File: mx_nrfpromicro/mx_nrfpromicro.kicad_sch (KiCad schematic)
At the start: 21 parts, among them J1 Conn_01x02, SW1 SW_Push_45deg, SW10 SW_Push_45deg, SW11 SW_Push_45deg, SW12 SW_Push_45deg, SW13 SW_Push_45deg, SW14 SW_Push_45deg, SW15 SW_Push_45deg, SW16 SW_Push_45deg, SW17 SW_Push_45deg, SW18 SW_Push, SW2 SW_Push_45deg, SW3 SW_Push_45deg, SW4 SW_Push_45deg, SW5 SW_Push_45deg, SW6 SW_Push_45deg, SW7 SW_Push_45deg, SW8 SW_Push_45deg, SW9 SW_Push_45deg, U1 Nice_Nano_V2

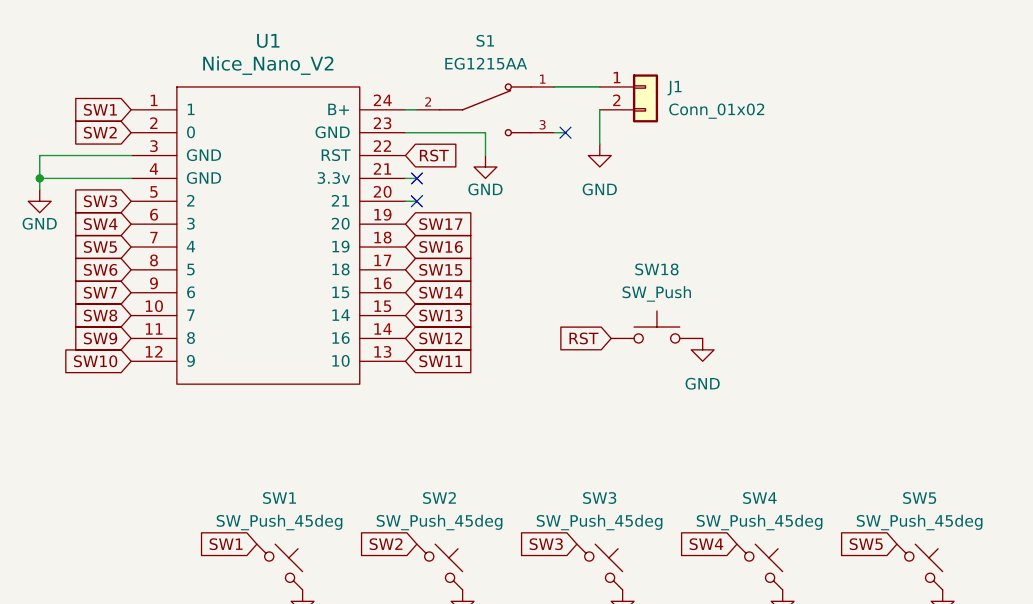
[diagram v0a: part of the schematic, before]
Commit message: updated
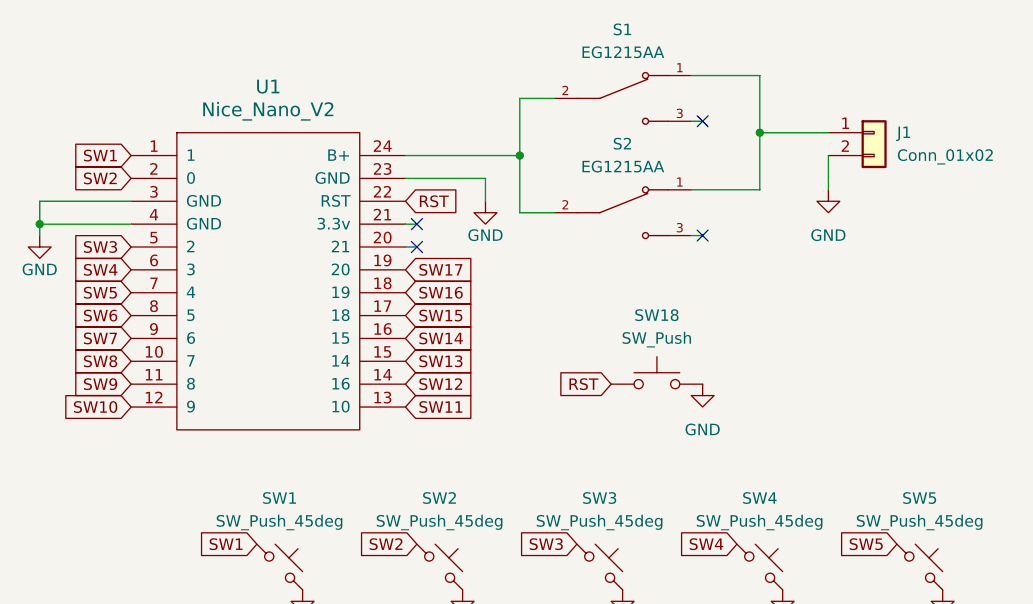
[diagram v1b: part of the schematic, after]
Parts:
- added S2: EG1215AA, EG1215AA:SW_EG1215AA, symbol EG1215AA:EG1215AA
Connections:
- net at S1.2, U1.24 (B+): now also S2.2
- net at J1.1 (Pin_1), S1.1: now also S2.1
- no-connect marks 3 -> 4
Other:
- moved on the sheet: J1, S1, SW18, U1

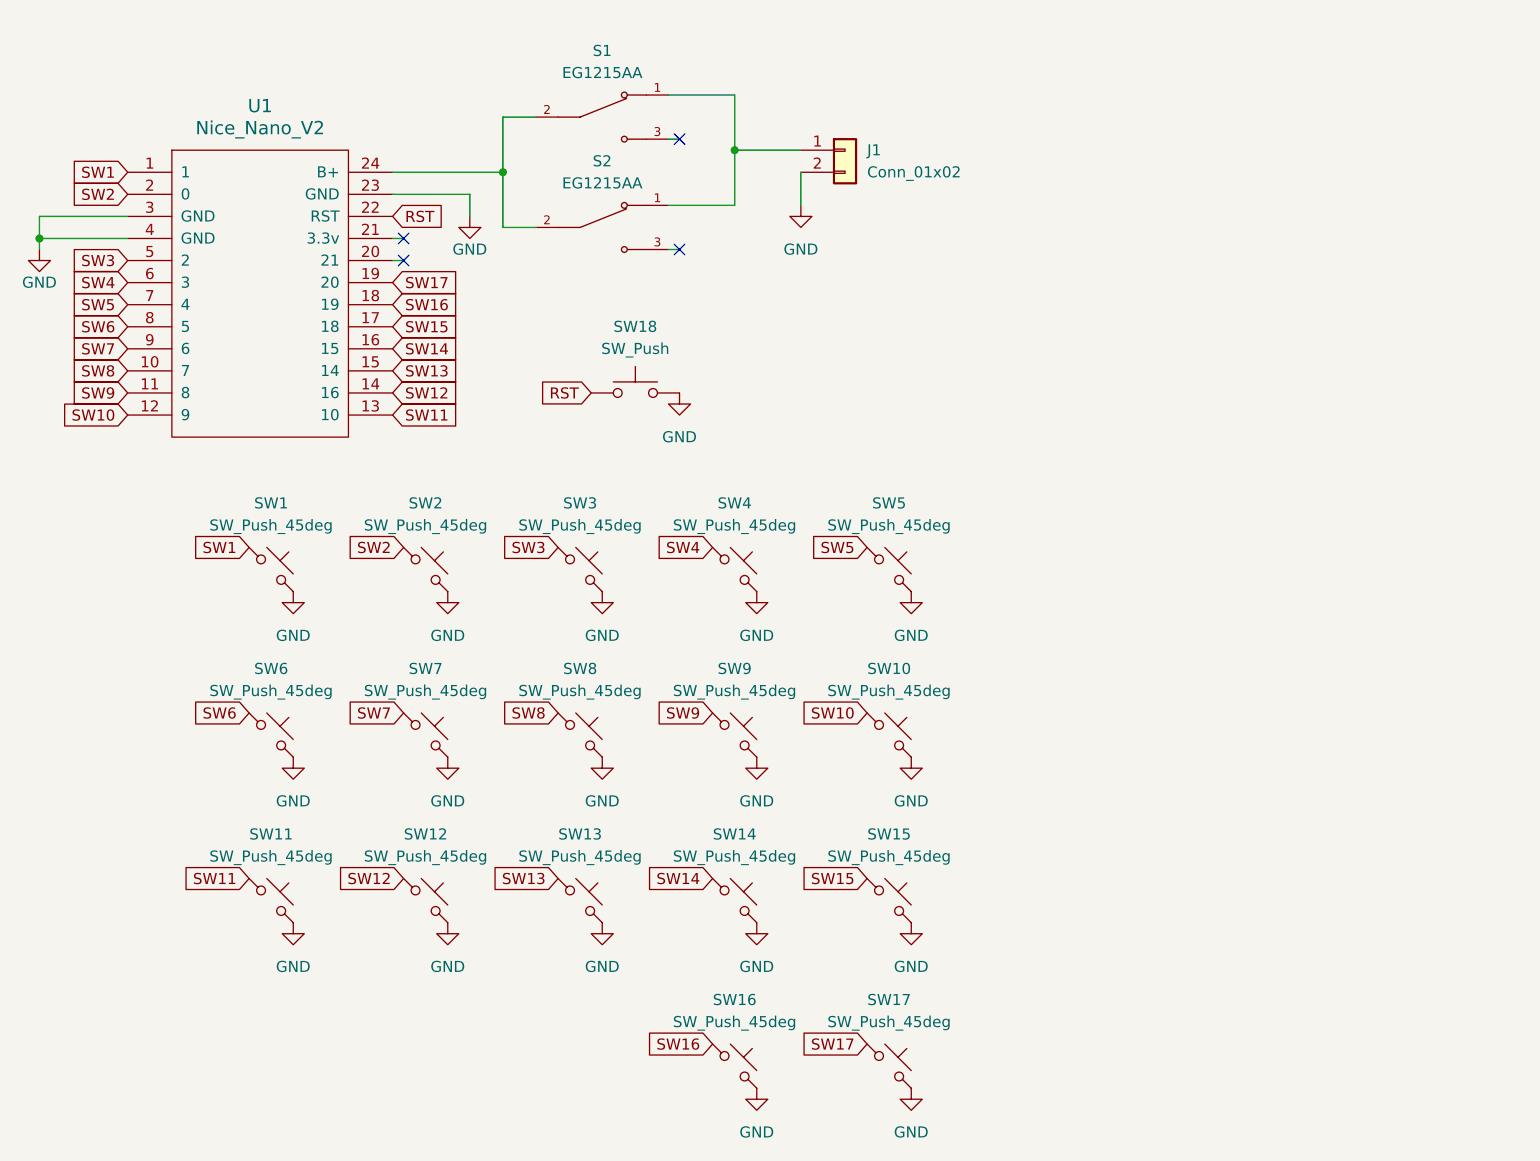
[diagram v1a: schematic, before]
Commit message: updated
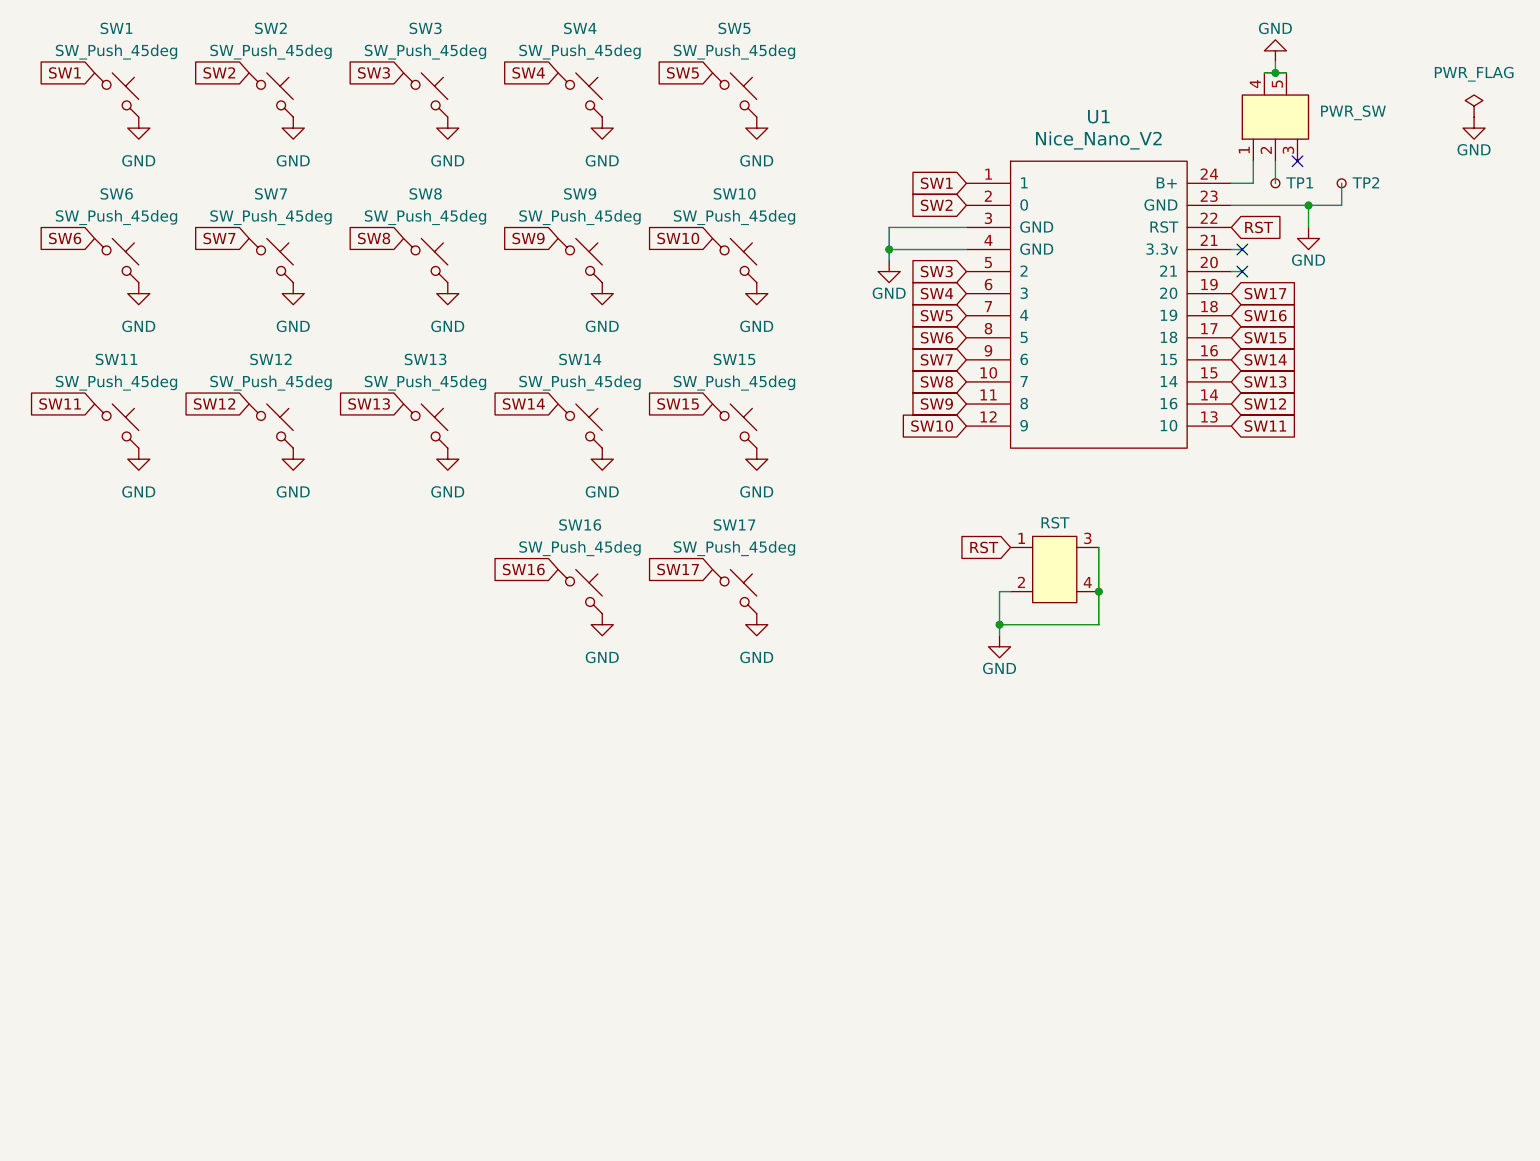
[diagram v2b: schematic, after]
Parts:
- removed J1: Conn_01x02, symbol Connector_Generic:Conn_01x02
- removed S1, S2: EG1215AA, EG1215AA:SW_EG1215AA, symbol EG1215AA:EG1215AA
- removed SW18: SW_Push, symbol Switch:SW_Push
- added PWR_SW: ~, BLE_KBD:SS12F23G5, symbol SS12F23G5:SS12F23G5
- added RST: ~, BLE_KBD:SW_SIDE_MOUNT, symbol SW_SIDE_MOUNT:SW_SIDE_MOUNT
- added TP1, TP2: TestPoint_Small, TestPoint:TestPoint_THTPad_D1.0mm_Drill0.5mm, symbol Connector:TestPoint_Small
- SW1, SW10, SW11, SW12, SW13, SW14, SW15, SW2, SW3, SW4, SW5, SW6, SW7, SW8, SW9: footprint (none) -> BLE_KBD:MX_Optional_Reversible_1u
- SW16, SW17: footprint (none) -> BLE_KBD:MX_Optional_Reversible_1.5u
- U1: footprint ScottoKeebs_MCU:Nice_Nano_V2 -> BLE_KBD:Nice_Nano_V2
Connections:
- net GND: now also PWR_SW.4, PWR_SW.5, RST.2, RST.3, RST.4, TP2.1
- net RST: now also RST.1
- net at U1.24 (B+): now also PWR_SW.1
- new net: PWR_SW.2, TP1.1
- no-connect marks 4 -> 3
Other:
- moved on the sheet: SW1, SW10, SW11, SW12, SW13, SW14, SW15, SW16, SW17, SW2, SW3, SW4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
